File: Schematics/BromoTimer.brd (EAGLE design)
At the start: 102.5 x 83.8 mm, 28 parts, among them IC1 PIC16F687, IC2 7805TV, K1 G2R2A, K2 G2R2A, Q1 BC548B, Q2 BC548B, Q3 BC548B, X1 AC_IN, X4 22-23-2031, X5 AC_OUT

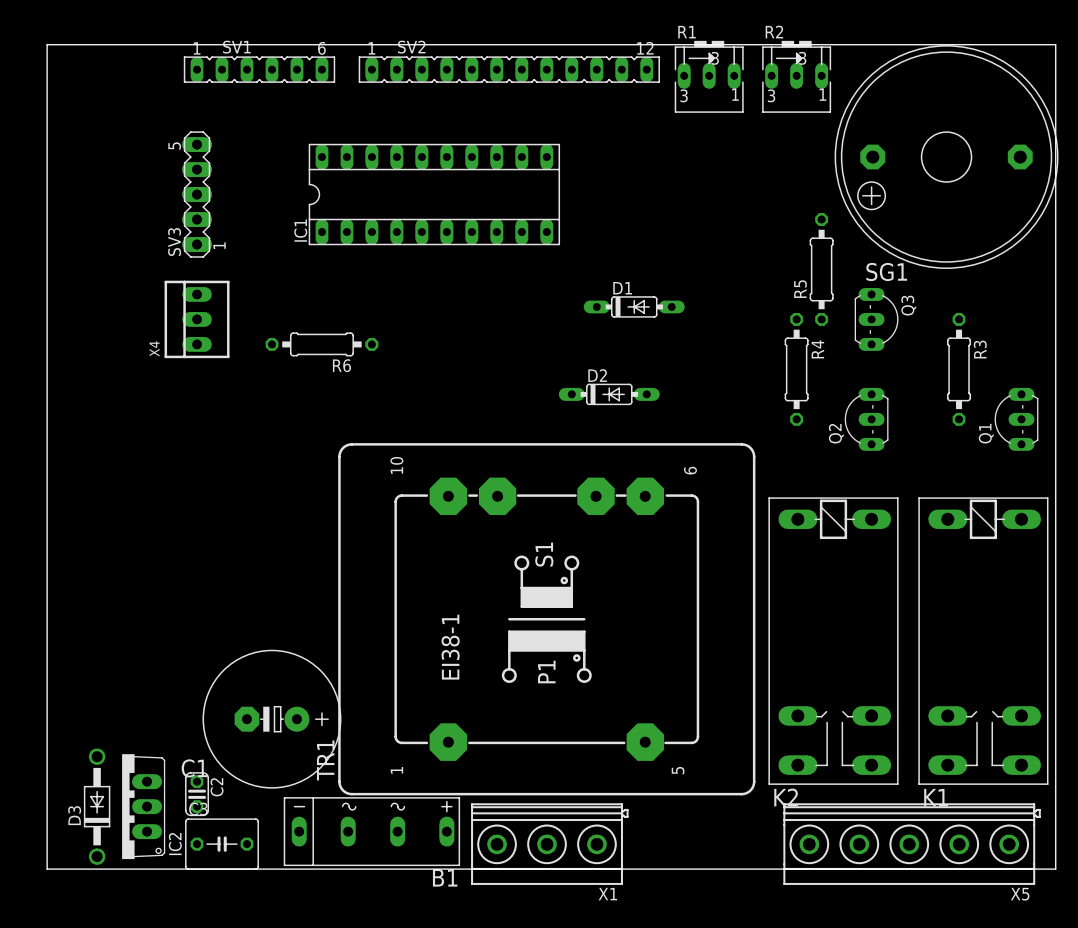
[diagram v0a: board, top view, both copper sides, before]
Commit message: Component placement finished
This is just a candidate though. The area with Q1 Q2 and Q3 could get optimized
a little more though...
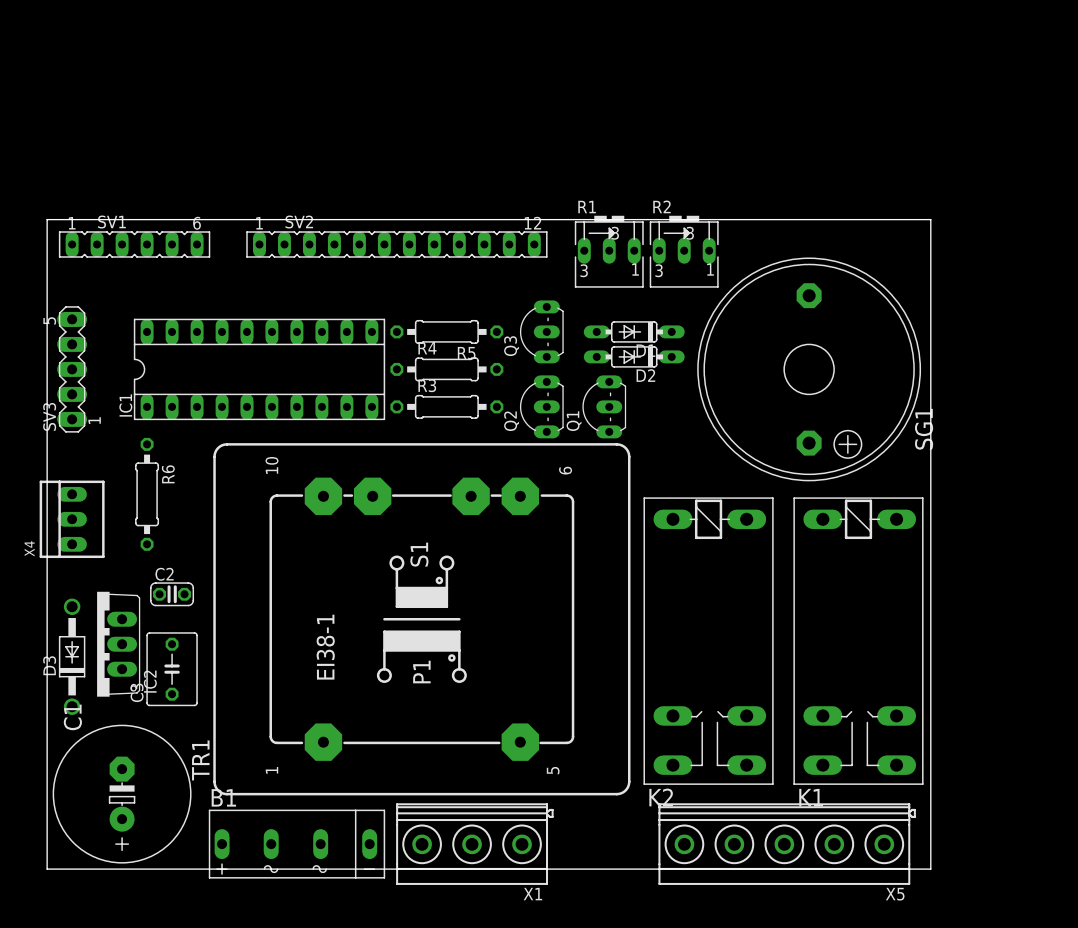
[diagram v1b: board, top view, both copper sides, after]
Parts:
- moved R3 52.2 mm to (40.6, 47.0), turned to 0 degrees
- moved Q1 41.9 mm to (55.9, 47.0)
- moved R5 38.6 mm to (40.6, 54.6), turned to 180 degrees
- moved Q3 35.6 mm to (49.5, 54.6), turned to 90 degrees
- moved R4 35.6 mm to (40.6, 50.8), turned to 0 degrees
- moved Q2 33.0 mm to (49.5, 47.0)
- moved SG1 25.7 mm to (77.5, 50.8), turned to 270 degrees
- moved IC1 25.1 mm to (21.6, 50.8)
- moved X4 24.0 mm to (2.54, 35.6)
- moved R6 23.4 mm to (10.2, 38.1), turned to 270 degrees
- moved SV1 21.8 mm to (8.89, 63.5)
- moved SV3 21.8 mm to (2.54, 50.8)
- moved R2 21.1 mm to (64.8, 62.2)
- moved SV2 21.1 mm to (35.6, 63.5)
- moved R1 20.5 mm to (57.1, 62.2)
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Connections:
- removed net N$22: TR1.5, X1.1
- net AC1: now also TR1.5, X1.1
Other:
- board size 102.5 x 83.8 mm -> 89.8 x 66 mm
